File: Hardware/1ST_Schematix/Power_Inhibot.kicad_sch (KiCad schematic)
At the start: 14 parts, among them J1 USB_C_Receptacle_USB2.0_16P, U2 BQ25896RTW, U3 LP2985-3.3

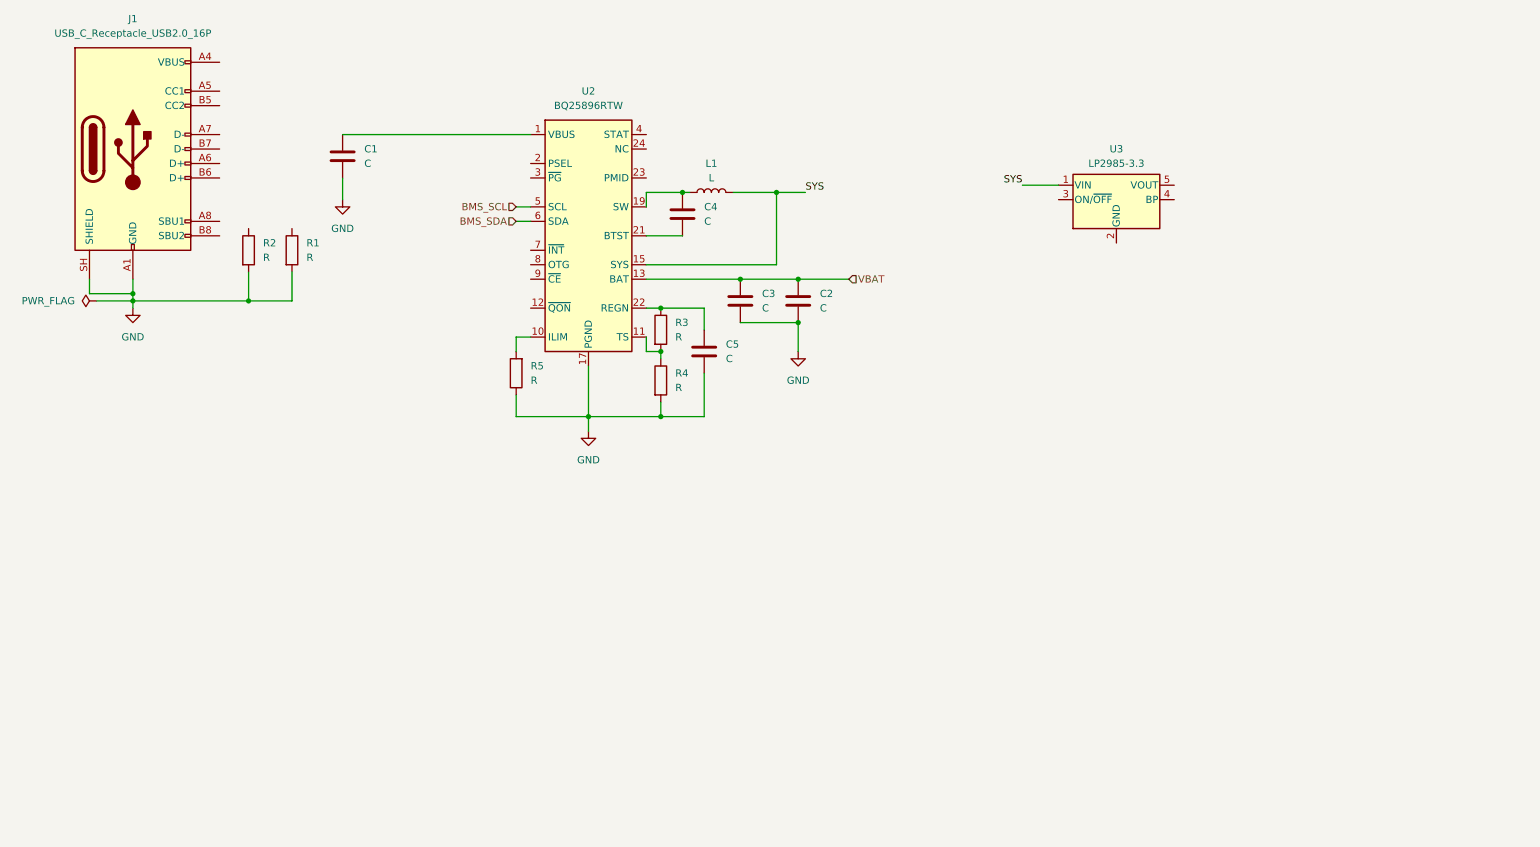
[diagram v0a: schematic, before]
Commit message: PCB POWER
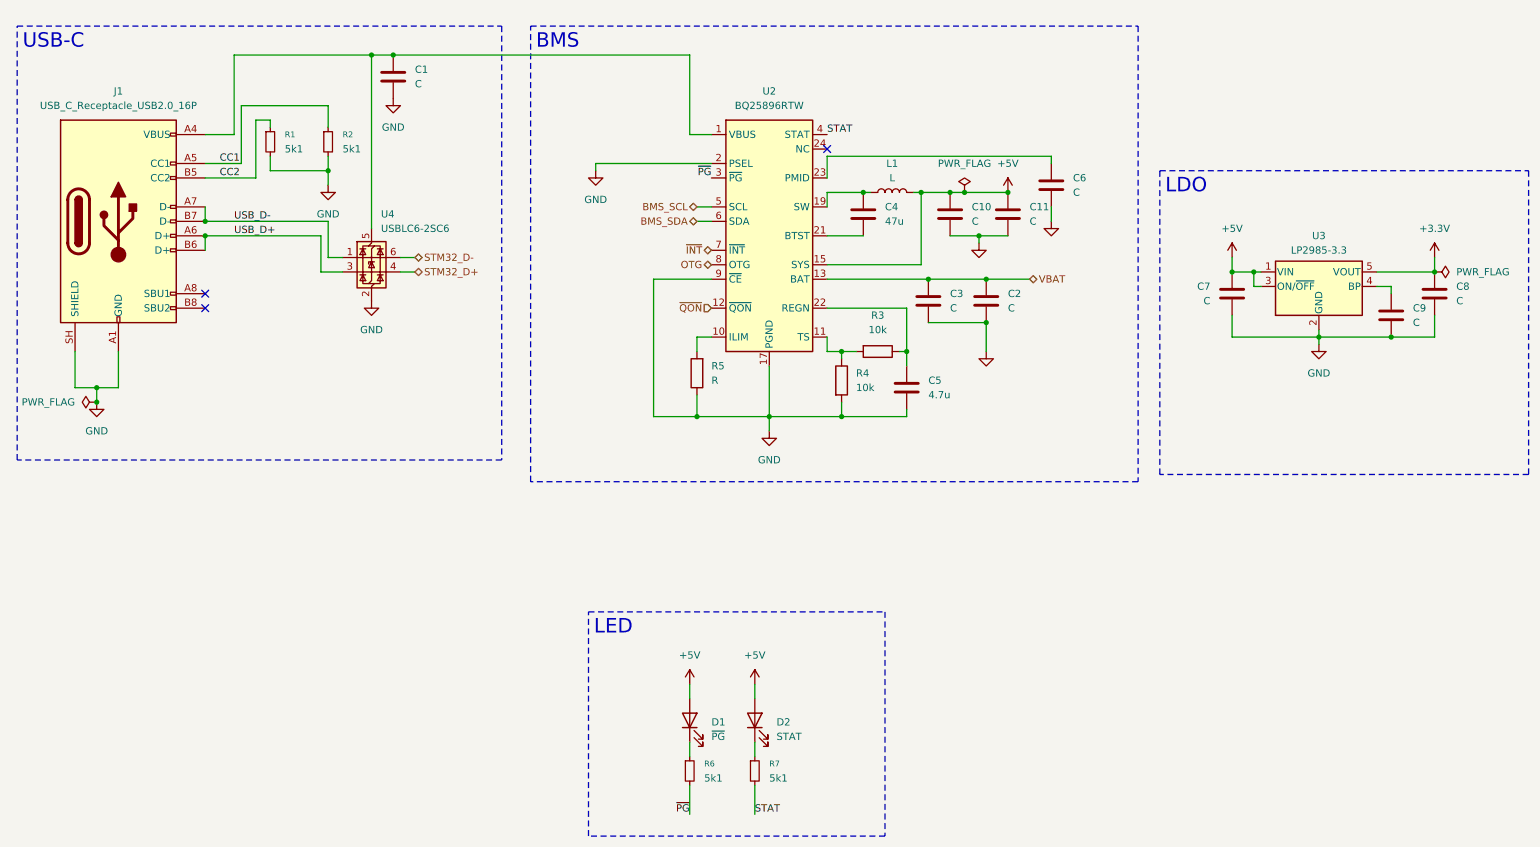
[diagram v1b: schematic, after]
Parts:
- removed R1, R2: R, symbol Device:R
- added C10, C11, C6, C7, C8, C9: C, symbol Device:C
- added D1: ~{PG}, Package_DFN_QFN:Texas_RTW_WQFN-24-1EP_4x4mm_P0.5mm_EP2.7x2.7mm_ThermalVias, symbol Device:LED
- added D2: STAT, Package_DFN_QFN:Texas_RTW_WQFN-24-1EP_4x4mm_P0.5mm_EP2.7x2.7mm_ThermalVias, symbol Device:LED
- added R1, R2, R6, R7: 5k1, Resistor_SMD:R_0402_1005Metric, symbol Device:R_Small
- added U4: USBLC6-2SC6, Package_TO_SOT_SMD:SOT-23-6, symbol Power_Protection:USBLC6-2SC6
- C4: value C -> 47u
- C5: value C -> 4.7u
- R3, R4: value R -> 10k
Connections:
- net SYS is gone; now on net +5V: L1.2, U2.15 (SYS), U2.16 (SYS), U3.1 (VIN)
- net GND: now also U2.2 (PSEL), U2.9 (~{CE}), U3.2 (GND), C10.2, C11.2, C6.2, C7.2, C8.2, C9.2, R1.2, R2.2, U4.2 (GND)
- net at J1.A4 (VBUS), J1.A9 (VBUS), J1.B4 (VBUS)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: now also C1.1, U2.1 (VBUS), U4.5 (VBUS)
- net CC1: now reaches J1.A5 (CC1)
- net CC1: now also R2.1
- net USB_D+: now reaches J1.A6 (D+)
- net USB_D+: now also J1.B6 (D+), U4.3 (I/O2)
- net USB_D-: now reaches J1.A7 (D-)
- net USB_D-: now also J1.B7 (D-), U4.1 (I/O1)
- net CC2: now reaches J1.B5 (CC2)
- net CC2: now also R1.1
- net ~{QON}: now reaches U2.12 (~{QON})
- net at U2.23 (PMID): now also C6.1
- net ~{PG}: now reaches U2.3 (~{PG})
- net ~{PG}: now also R6.2
- net STAT: now reaches U2.4 (STAT)
- net STAT: now also R7.2
- net ~{INT}: now reaches U2.7 (~{INT})
- net OTG: now reaches U2.8 (OTG)
- net +5V: now reaches U3.3 (ON/~{OFF})
- net +5V: now also C10.1, C11.1, C7.1, D1.2 (A), D2.2 (A)
- net at U3.4 (BP): now also C9.1
- net +3.3V: now reaches U3.5 (VOUT)
- net +3.3V: now also C8.1
- new net: D2.1 (K), R7.1
- new net: D1.1 (K), R6.1
- new net STM32_D+: U4.4 (I/O2)
- new net STM32_D-: U4.6 (I/O1)
- no-connect marks 0 -> 3
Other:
- moved on the sheet: C1, C2, C3, C4, C5, J1, L1, R3, R4, R5, U2, U3
